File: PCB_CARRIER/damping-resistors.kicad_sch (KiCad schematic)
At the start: 0 parts

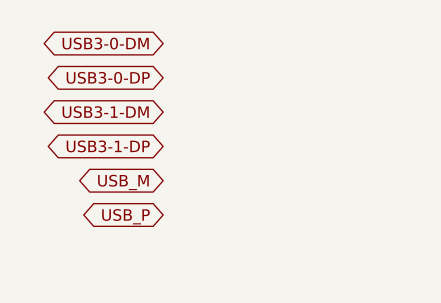
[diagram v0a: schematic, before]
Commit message: terminations on USB M/P
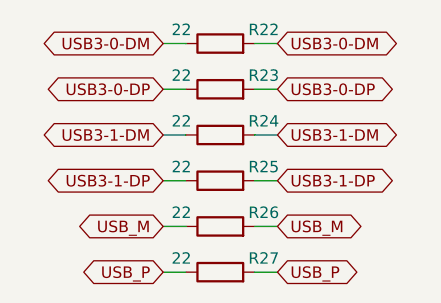
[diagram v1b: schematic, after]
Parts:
- added R22, R23, R24, R25, R26, R27: 22, symbol Device:R
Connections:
- net USB3-0-DM: now also R22.1, R22.2
- net USB3-0-DP: now also R23.1, R23.2
- net USB3-1-DM: now also R24.1, R24.2
- net USB3-1-DP: now also R25.1, R25.2
- net USB_M: now also R26.1, R26.2
- net USB_P: now also R27.1, R27.2
